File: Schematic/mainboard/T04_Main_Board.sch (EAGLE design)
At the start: 29 parts, among them IC1 7805DT, J1 AVR_SPI_PRG_6PTH, U1 ATMEGA328P_PDIP, X1 22-23-2021, X3 22-23-2081, Y1 16MHZ

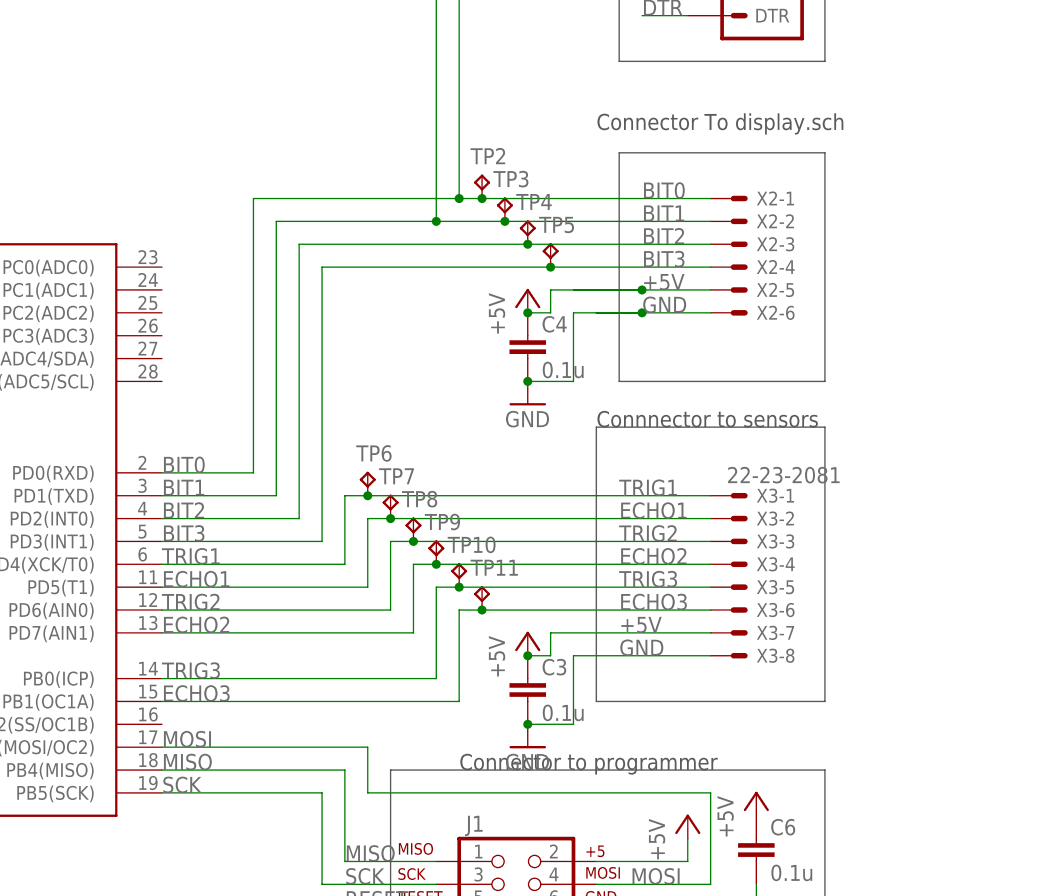
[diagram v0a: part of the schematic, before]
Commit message: M@INb0@RD C0MPl37e
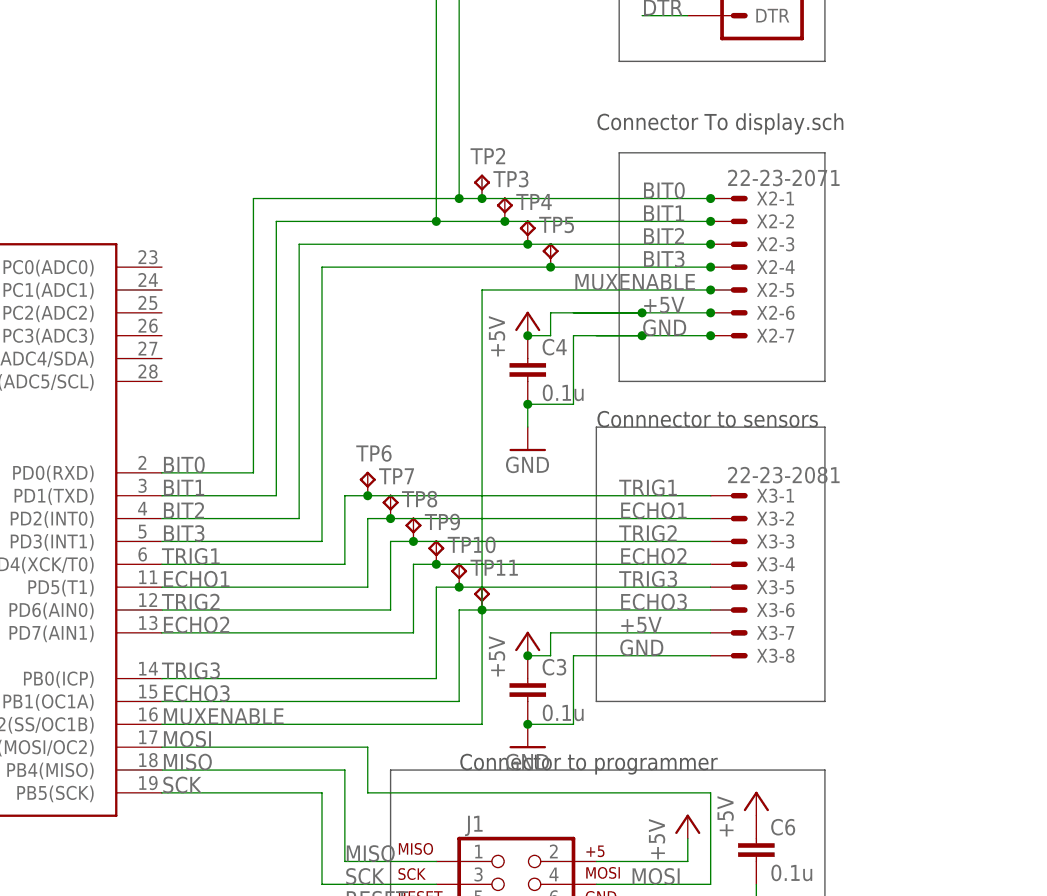
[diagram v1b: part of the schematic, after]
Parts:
- X2: value (none) -> 22-23-2071; device con-molex:22-23-2061 -> con-molex:22-23-2071
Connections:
- new net MUXENABLE: U1.PB2(SS/OC1B), X2-5.S
- net +5V: now also X2-6.S; no longer X2-5.S
- net GND: now also X2-7.S; no longer X2-6.S
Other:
- moved on the sheet: C4
